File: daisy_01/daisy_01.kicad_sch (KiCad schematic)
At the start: 18 parts, among them J1 AudioInput, J2 AudioOutput1, J3 AudioOutput2, Q1 PN2222A, SW1 SW_SPST, SW2 RotaryEncoder_Switch

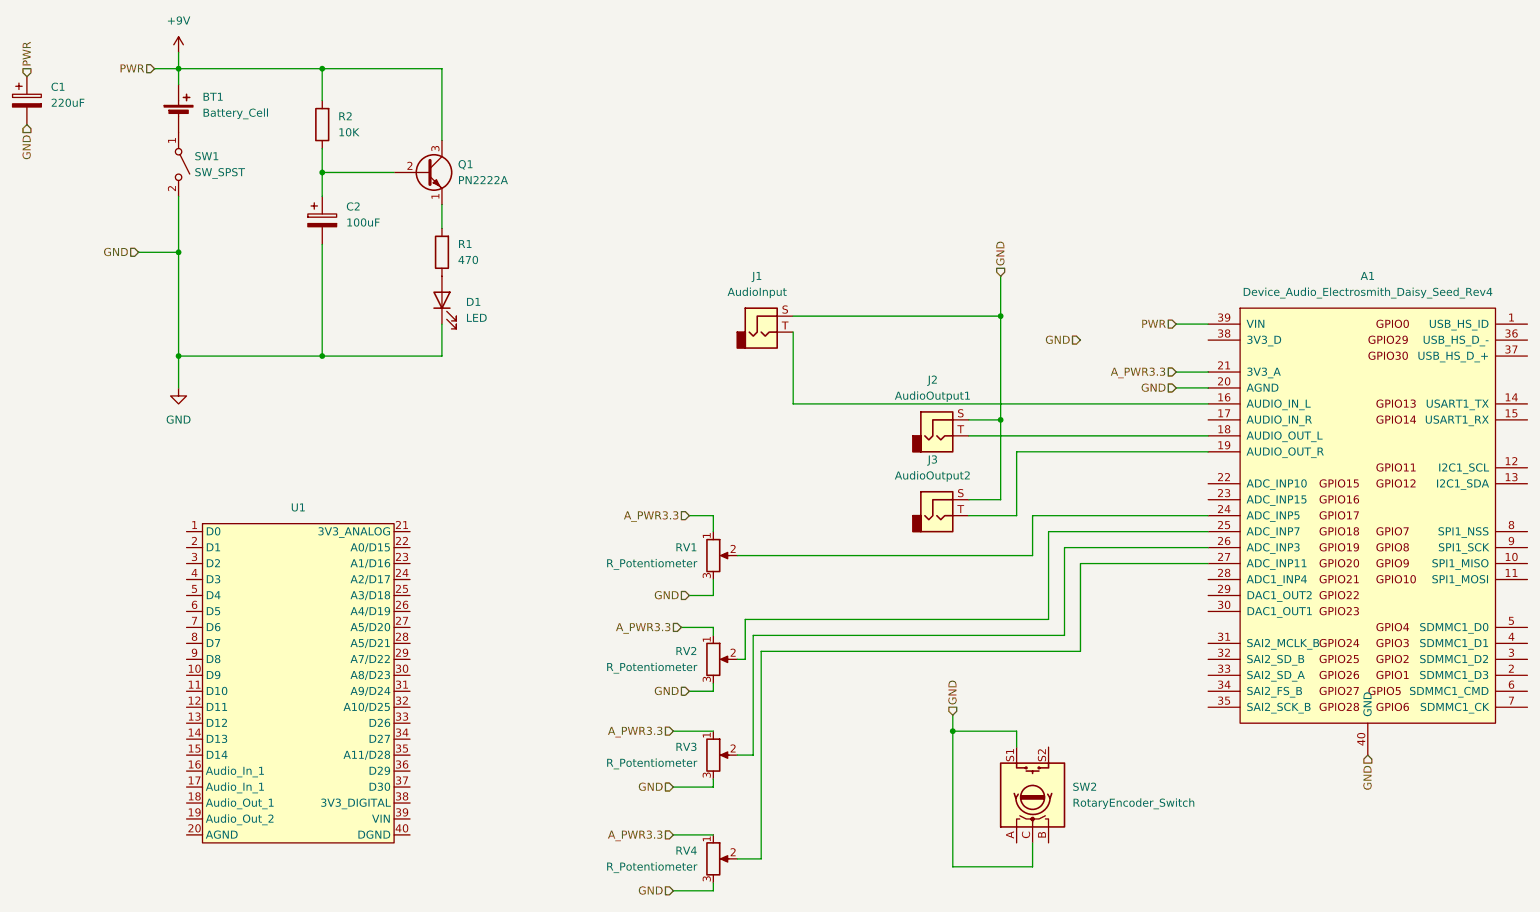
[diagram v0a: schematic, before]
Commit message: update
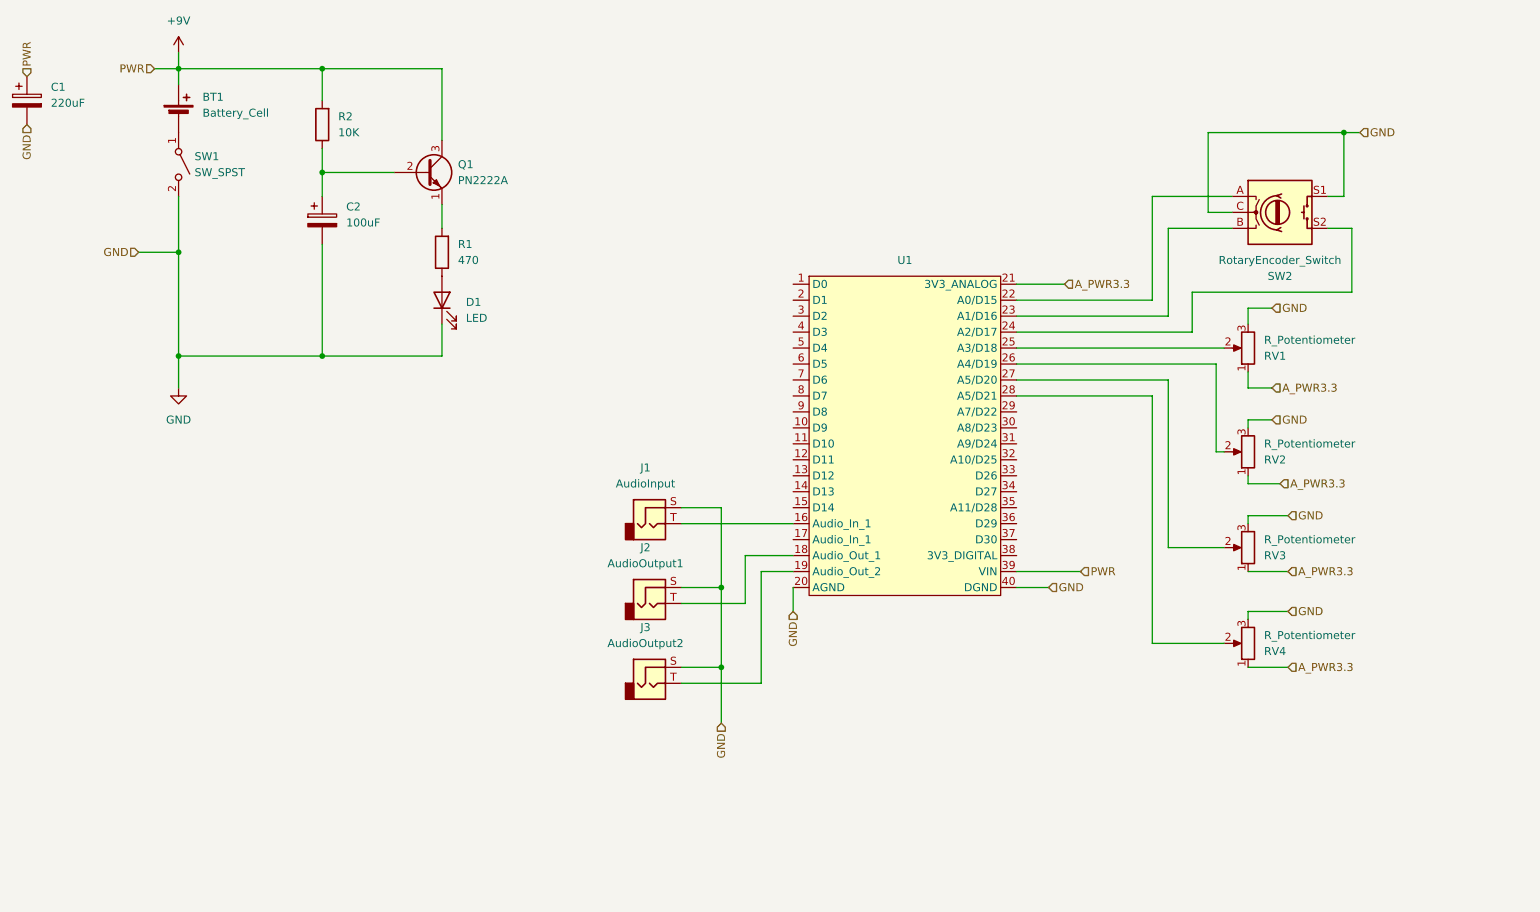
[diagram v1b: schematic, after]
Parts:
- removed A1: Device_Audio_Electrosmith_Daisy_Seed_Rev4, Daisy_Electrosmith:Device_Audio_Electrosmith_Daisy_Seed, symbol test_daisy:Device_Audio_Electrosmith_Daisy_Seed_Rev4
- SW2: footprint (none) -> Rotary_Encoder:RotaryEncoder_Alps_EC11E-Switch_Vertical_H20mm
- U1: footprint (none) -> Library_electrosmith:Device_Audio_Electrosmith_Daisy_Seed
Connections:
- net +9V: now also U1.39 (VIN)
- net A_PWR3.3: now also U1.21 (3V3_ANALOG)
- net GND: now also U1.20 (AGND), U1.40 (DGND)
- net at J1.T: now also U1.16 (Audio_In_1)
- net at J2.T: now also U1.18 (Audio_Out_1)
- net at J3.T: now also U1.19 (Audio_Out_2)
- net at RV1.2: now also U1.25 (A3/D18)
- net at RV2.2: now also U1.26 (A4/D19)
- net at RV3.2: now also U1.27 (A5/D20)
- net at RV4.2: now also U1.28 (A5/D21)
- net at SW2.A: now also U1.22 (A0/D15)
- net at SW2.B: now also U1.23 (A1/D16)
- net at SW2.S2: now also U1.24 (A2/D17)
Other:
- moved on the sheet: J1, J2, J3, RV1, RV2, RV3, RV4, SW2, U1
